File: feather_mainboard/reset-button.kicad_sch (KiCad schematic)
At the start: 4 parts

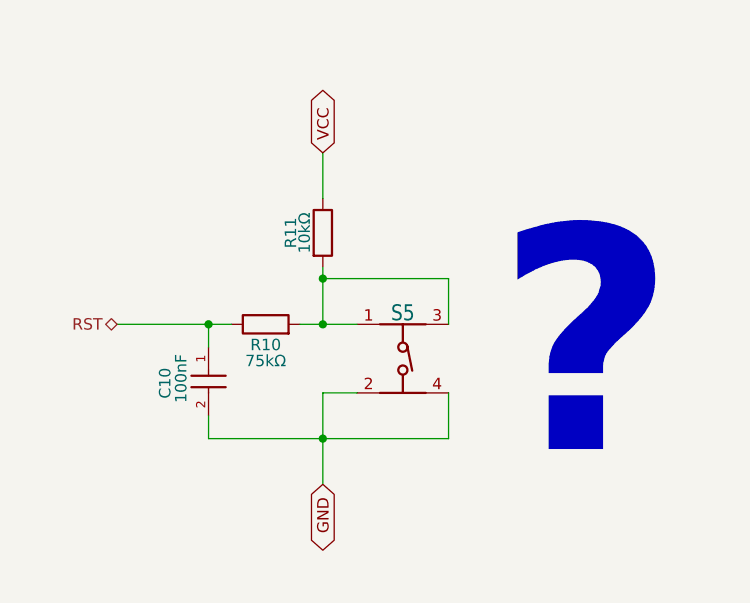
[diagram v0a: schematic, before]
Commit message: finished mainboard design, need to do the routing
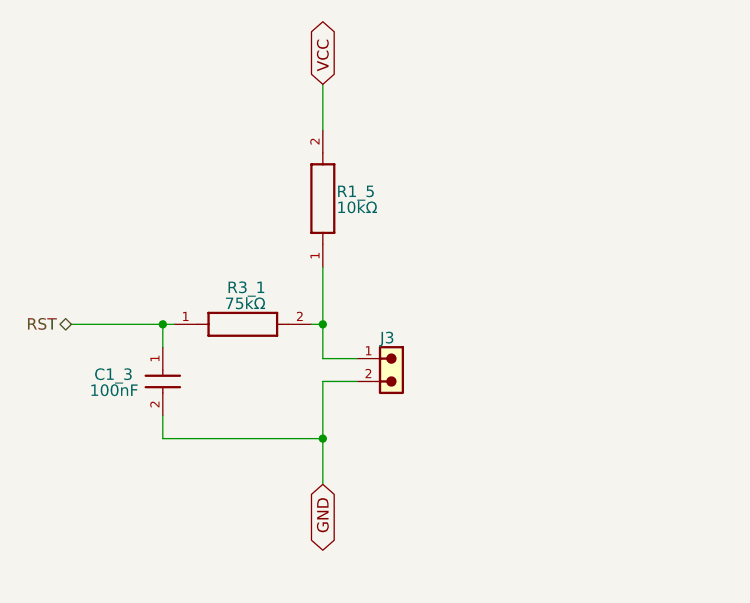
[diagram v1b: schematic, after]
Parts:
- removed C10: 100nF, Custom footprints:WCAP-CSGP_1210_H2.0, symbol WCAP-CSGP_1210_H2.0:WCAP-CSGP_1210_H2.0
- removed R10: 75kΩ, Resistor_SMD:R_0805_2012Metric_Pad1.20x1.40mm_HandSolder, symbol Device:R
- removed R11: 10kΩ, Resistor_SMD:R_0805_2012Metric_Pad1.20x1.40mm_HandSolder, symbol Device:R
- removed S5: 430182050816, Custom footprints:430182050816, symbol Projektarbeit_button:430182050816
- added C1_3: 100nF, Custom footprints:WCAP-CSGP_0603_R, symbol WCAP-CSGP_0603:WCAP-CSGP_0603
- added J3: 61300211121, Custom footprints:61300211121, symbol 6130XX11121_61300211121:6130XX11121_61300211121
- added R1_5: 10kΩ, Custom footprints:WRIS-RSKS_0603_REFLOW, symbol WRIS-RSKS_0603:WRIS-RSKS_0603
- added R3_1: 75kΩ, Custom footprints:WRIS-RSKS_0603_REFLOW, symbol WRIS-RSKS_0603:WRIS-RSKS_0603
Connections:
- net GND: now also C1_3.2, J3.2
- net RST: now also C1_3.1, R3_1.1
- net VCC: now also R1_5.2
- new net: J3.1, R1_5.1, R3_1.2
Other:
- note removed: "?"
